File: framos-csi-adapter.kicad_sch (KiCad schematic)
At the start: 66 parts, among them J1 Socket_Hirose_DF40_2x30_DF40C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, J2 Conn_STM_MSAK24025P30, U1 NTS0102_XSON, U2 AP62301Z6-7, U3 AP62301Z6-7

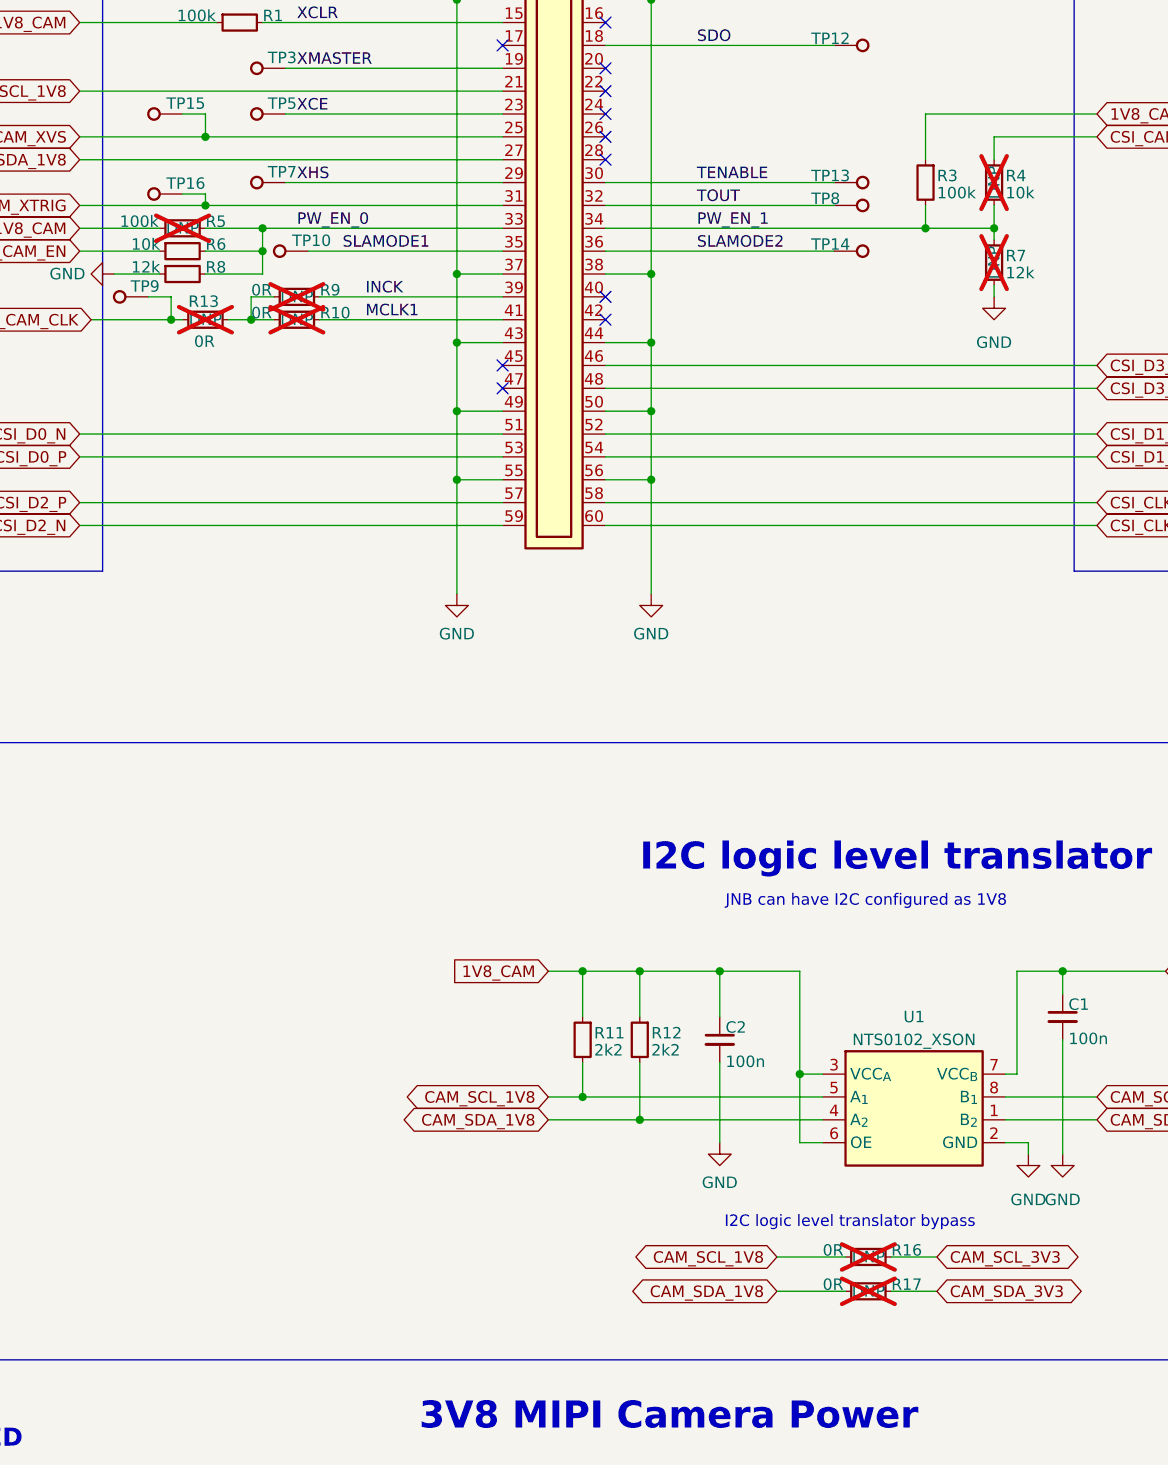
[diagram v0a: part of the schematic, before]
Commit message: [#74670] Perform DNP check
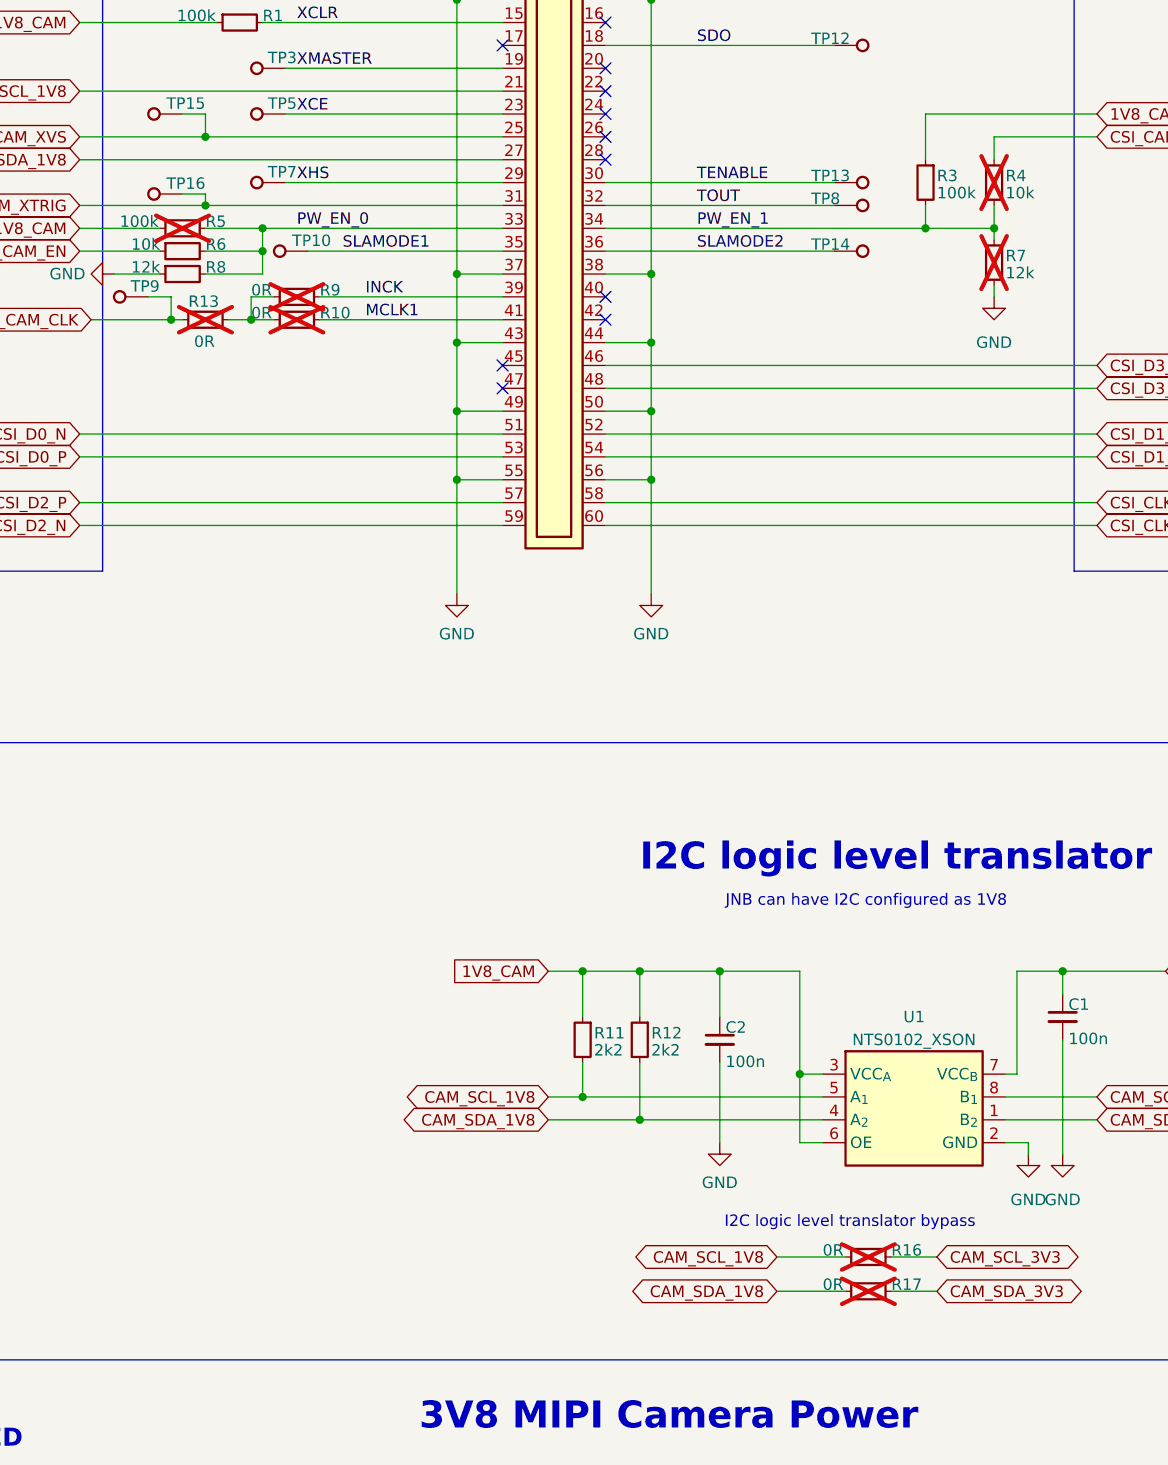
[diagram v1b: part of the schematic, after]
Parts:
- R10, R13, R16, R17, R4, R5, R7, R9: DNP DNP -> (none)
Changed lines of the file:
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@@
 			)
 		)
-		(property "DNP" "DNP"
-			(at 80.01 100.33 0)
-			(effects
-				(font
-					(size 1.27 1.27)
-				)
-			)
-		)
 		(property "License" "Apache-2.0"
 			(at 97.79 125.73 0)
@@
 			)
 		)
-		(property "DNP" "DNP"
-			(at 80.01 102.87 0)
-			(effects
-				(font
-					(size 1.27 1.27)
-				)
-			)
-		)
 		(property "License" "Apache-2.0"
 			(at 97.79 128.27 0)
@@
 			)
 		)
-		(property "DNP" "DNP"
-			(at 157.48 87.63 0)
-			(effects
-				(font
-					(size 1.27 1.27)
-				)
-			)
-		)
 		(property "License" "Apache-2.0"
 			(at 132.08 105.41 0)
@@
 			)
 		)
-		(property "DNP" "DNP"
-			(at 157.48 96.52 0)
-			(effects
-				(font
-					(size 1.27 1.27)
-				)
-			)
-		)
 		(property "License" "Apache-2.0"
 			(at 132.08 114.3 0)
@@
 			)
 		)
-		(property "DNP" "DNP"
-			(at 67.31 92.71 0)
-			(effects
-				(font
-					(size 1.27 1.27)
-				)
-			)
-		)
 		(property "License" "Apache-2.0"
 			(at 85.09 118.11 0)
@@
 			)
 		)
-		(property "DNP" "DNP"
-			(at 143.51 210.82 0)
-			(effects
-				(font
-					(size 1.27 1.27)
-				)
-			)
-		)
 		(property "License" "Apache-2.0"
 			(at 161.29 236.22 0)
@@
 			)
 		)
-		(property "DNP" "DNP"
-			(at 143.51 207.01 0)
-			(effects
-				(font
-					(size 1.27 1.27)
-				)
-			)
-		)
 		(property "License" "Apache-2.0"
 			(at 161.29 232.41 0)
@@
 			)
 		)
-		(property "DNP" "DNP"
-			(at 69.85 102.87 0)
-			(effects
-				(font
-					(size 1.27 1.27)
-				)
-			)
-		)
